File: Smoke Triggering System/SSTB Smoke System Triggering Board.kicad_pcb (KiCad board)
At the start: 2 copper layers, 87.6 x 27.9 mm, 12 parts, among them J1 Conn_01x02, J2 Conn_01x06, J3 8P8C, U1 PIC16LF18325-ISL, U2 LP2985-5.0

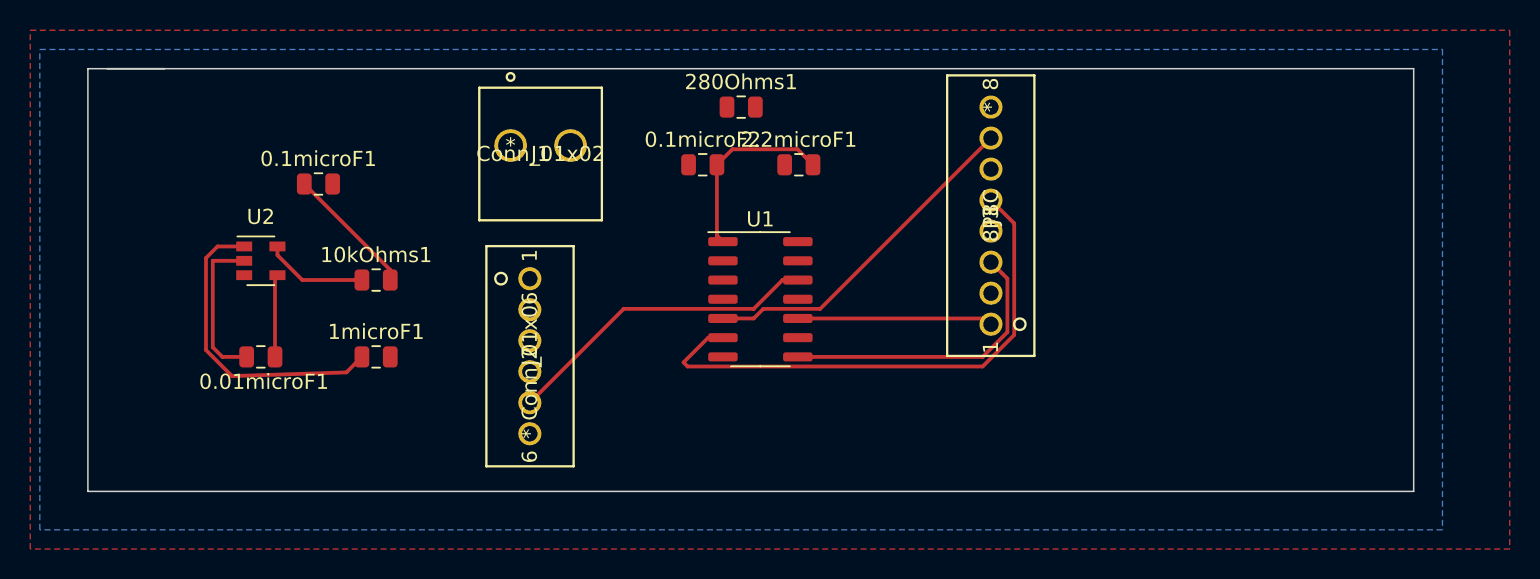
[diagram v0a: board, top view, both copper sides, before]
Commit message: inital commit
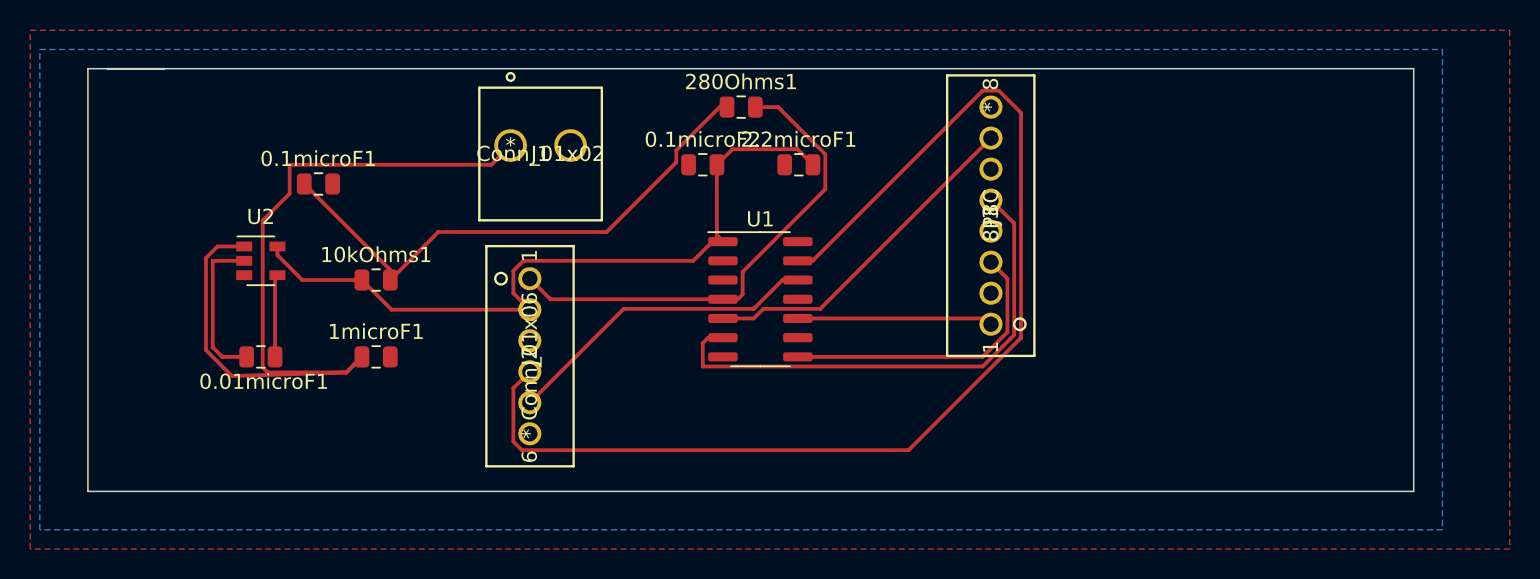
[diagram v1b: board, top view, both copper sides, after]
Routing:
- net ICSPDAT: track 0.00 -> 76.8 mm
- net 9V: track 20.4 -> 56.8 mm
- net MCLR: track 0.00 -> 32.2 mm
- net +3V3: track 19.3 -> 49.1 mm
- net Net-(0.1microF1-Pad1): track 8.70 -> 36.2 mm
- net Net-(J3-Pad5): track 35.7 -> 34.0 mm
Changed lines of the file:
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@@
     (thickness 1.6)
     (drawings 5)
-    (tracks 49)
+    (tracks 91)
     (zones 0)
     (modules 12)
@@
   (segment (start 140.6375 103.475) (end 140.6375 104.14) (width 0.25) (layer F.Cu) (net 3))
   (segment (start 134.9525 97.79) (end 140.6375 103.475) (width 0.25) (layer F.Cu) (net 3))
+  (segment (start 140.6375 104.14) (end 143.8125 100.965) (width 0.25) (layer F.Cu) (net 3))
+  (segment (start 143.8125 100.965) (end 154.94 100.965) (width 0.25) (layer F.Cu) (net 3))
+  (segment (start 162.405 92.71) (end 162.8925 92.71) (width 0.25) (layer F.Cu) (net 3))
+  (segment (start 159.53999 95.57501) (end 162.405 92.71) (width 0.25) (layer F.Cu) (net 3))
+  (segment (start 154.94 100.965) (end 159.53999 96.36501) (width 0.25) (layer F.Cu) (net 3))
+  (segment (start 159.53999 96.36501) (end 159.53999 95.57501) (width 0.25) (layer F.Cu) (net 3))
   (segment (start 167.55249 95.49499) (end 168.091973 96.034473) (width 0.25) (layer F.Cu) (net 4))
   (segment (start 168.091973 96.034473) (end 168.5775 96.52) (width 0.25) (layer F.Cu) (net 4))
@@
   (segment (start 138.275 104.14) (end 138.7625 104.14) (width 0.25) (layer F.Cu) (net 4))
   (segment (start 133.18 101.92) (end 133.18 102.495) (width 0.25) (layer F.Cu) (net 4))
+  (segment (start 140.7225 106.1) (end 149.86 106.1) (width 0.25) (layer F.Cu) (net 4))
+  (segment (start 138.7625 104.14) (end 140.7225 106.1) (width 0.25) (layer F.Cu) (net 4))
+  (segment (start 148.772999 103.528238) (end 149.431237 102.87) (width 0.25) (layer F.Cu) (net 4))
+  (segment (start 149.86 106.1) (end 148.772999 105.012999) (width 0.25) (layer F.Cu) (net 4))
+  (segment (start 148.772999 105.012999) (end 148.772999 103.528238) (width 0.25) (layer F.Cu) (net 4))
+  (segment (start 149.431237 102.87) (end 160.655 102.87) (width 0.25) (layer F.Cu) (net 4))
+  (segment (start 162.325 101.3) (end 162.625 101.6) (width 0.25) (layer F.Cu) (net 4))
+  (segment (start 162.225 101.3) (end 162.325 101.3) (width 0.25) (layer F.Cu) (net 4))
+  (segment (start 160.655 102.87) (end 162.225 101.3) (width 0.25) (layer F.Cu) (net 4))
+  (segment (start 151.220001 105.41) (end 162.625 105.41) (width 0.25) (layer F.Cu) (net 5))
+  (segment (start 149.86 104.049999) (end 151.220001 105.41) (width 0.25) (layer F.Cu) (net 5))
+  (segment (start 163.92501 105.08499) (end 163.6 105.41) (width 0.25) (layer F.Cu) (net 5))
+  (segment (start 169.39001 98.138222) (end 163.92501 103.603222) (width 0.25) (layer F.Cu) (net 5))
+  (segment (start 163.6 105.41) (end 162.625 105.41) (width 0.25) (layer F.Cu) (net 5))
+  (segment (start 169.39001 95.82816) (end 169.39001 98.138222) (width 0.25) (layer F.Cu) (net 5))
+  (segment (start 166.27185 92.71) (end 169.39001 95.82816) (width 0.25) (layer F.Cu) (net 5))
+  (segment (start 163.92501 103.603222) (end 163.92501 105.08499) (width 0.25) (layer F.Cu) (net 5))
+  (segment (start 164.7675 92.71) (end 166.27185 92.71) (width 0.25) (layer F.Cu) (net 5))
   (segment (start 138.276973 109.705527) (end 138.7625 109.22) (width 0.25) (layer F.Cu) (net 6))
   (segment (start 137.73749 110.24501) (end 138.276973 109.705527) (width 0.25) (layer F.Cu) (net 6))
@@
   (segment (start 129.21859 101.92) (end 128.45499 102.6836) (width 0.25) (layer F.Cu) (net 6))
   (segment (start 130.98 101.92) (end 129.21859 101.92) (width 0.25) (layer F.Cu) (net 6))
+  (segment (start 138.7625 109.22) (end 137.73749 110.24501) (width 0.25) (layer F.Cu) (net 6))
+  (segment (start 147.32 96.52) (end 148.59 95.25) (width 0.25) (layer F.Cu) (net 6))
+  (segment (start 133.985 96.52) (end 147.32 96.52) (width 0.25) (layer F.Cu) (net 6))
+  (segment (start 132.53816 110.24501) (end 132.20499 109.91184) (width 0.25) (layer F.Cu) (net 6))
+  (segment (start 133.985 98.425) (end 133.985 96.52) (width 0.25) (layer F.Cu) (net 6))
+  (segment (start 137.73749 110.24501) (end 132.53816 110.24501) (width 0.25) (layer F.Cu) (net 6))
+  (segment (start 132.20499 109.91184) (end 132.20499 100.20501) (width 0.25) (layer F.Cu) (net 6))
+  (segment (start 132.20499 100.20501) (end 133.985 98.425) (width 0.25) (layer F.Cu) (net 6))
   (segment (start 166.561822 104.14) (end 166.6 104.14) (width 0.25) (layer F.Cu) (net 8))
   (segment (start 164.656822 106.045) (end 166.561822 104.14) (width 0.25) (layer F.Cu) (net 8))
@@
   (segment (start 166.6 104.14) (end 167.575 104.14) (width 0.25) (layer F.Cu) (net 8))
   (segment (start 149.86 112.25) (end 156.065 106.045) (width 0.25) (layer F.Cu) (net 8))
+  (segment (start 179.797001 91.622999) (end 168.55 102.87) (width 0.25) (layer F.Cu) (net 9))
+  (segment (start 180.861761 91.622999) (end 179.797001 91.622999) (width 0.25) (layer F.Cu) (net 9))
+  (segment (start 182.327021 107.954561) (end 182.327021 93.088259) (width 0.25) (layer F.Cu) (net 9))
+  (segment (start 174.894582 115.387) (end 182.327021 107.954561) (width 0.25) (layer F.Cu) (net 9))
+  (segment (start 149.338239 115.387) (end 174.894582 115.387) (width 0.25) (layer F.Cu) (net 9))
+  (segment (start 148.772999 114.82176) (end 149.338239 115.387) (width 0.25) (layer F.Cu) (net 9))
+  (segment (start 182.327021 93.088259) (end 180.861761 91.622999) (width 0.25) (layer F.Cu) (net 9))
+  (segment (start 148.772999 111.287) (end 148.772999 114.82176) (width 0.25) (layer F.Cu) (net 9))
+  (segment (start 168.55 102.87) (end 167.575 102.87) (width 0.25) (layer F.Cu) (net 9))
+  (segment (start 149.86 110.199999) (end 148.772999 111.287) (width 0.25) (layer F.Cu) (net 9))
   (segment (start 164.658232 106.68) (end 165.293232 106.045) (width 0.25) (layer F.Cu) (net 12))
   (segment (start 162.625 106.68) (end 164.658232 106.68) (width 0.25) (layer F.Cu) (net 12))
   (segment (start 169.055001 106.045) (end 180.34 94.760001) (width 0.25) (layer F.Cu) (net 12))
   (segment (start 165.293232 106.045) (end 169.055001 106.045) (width 0.25) (layer F.Cu) (net 12))
-  (segment (start 161.65 107.95) (end 160.02 109.58) (width 0.25) (layer F.Cu) (net 13))
   (segment (start 162.625 107.95) (end 161.65 107.95) (width 0.25) (layer F.Cu) (net 13))
-  (segment (start 160.02 109.58) (end 160.295 109.855) (width 0.25) (layer F.Cu) (net 13))
-  (segment (start 160.295 109.855) (end 179.790172 109.855) (width 0.25) (layer F.Cu) (net 13))
   (segment (start 179.790172 109.855) (end 181.877011 107.768161) (width 0.25) (layer F.Cu) (net 13))
   (segment (start 181.877011 100.397012) (end 180.34 98.860001) (width 0.25) (layer F.Cu) (net 13))
   (segment (start 181.877011 107.768161) (end 181.877011 100.397012) (width 0.25) (layer F.Cu) (net 13))
+  (segment (start 161.29 108.31) (end 161.65 107.95) (width 0.25) (layer F.Cu) (net 13))
+  (segment (start 161.29 109.855) (end 161.29 108.31) (width 0.25) (layer F.Cu) (net 13))
+  (segment (start 161.29 109.855) (end 179.790172 109.855) (width 0.25) (layer F.Cu) (net 13))
   (segment (start 181.101999 103.721999) (end 180.34 102.96) (width 0.25) (layer F.Cu) (net 14))
   (segment (start 181.427001 104.047001) (end 181.101999 103.721999) (width 0.25) (layer F.Cu) (net 14))
